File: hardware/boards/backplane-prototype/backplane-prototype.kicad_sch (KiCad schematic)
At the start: 16 parts, among them J1 DC_IN, J10 SLOT_3_IO, J11 SLOT_4_IO, J12 SLOT_5_IO, J13 SLOT_6_IO, J2 SLOT_1, J3 SLOT_2, J4 SLOT_3, J5 SLOT_4, J6 SLOT_5, J7 SLOT_6, J8 SLOT_1_IO, J9 SLOT_2_IO

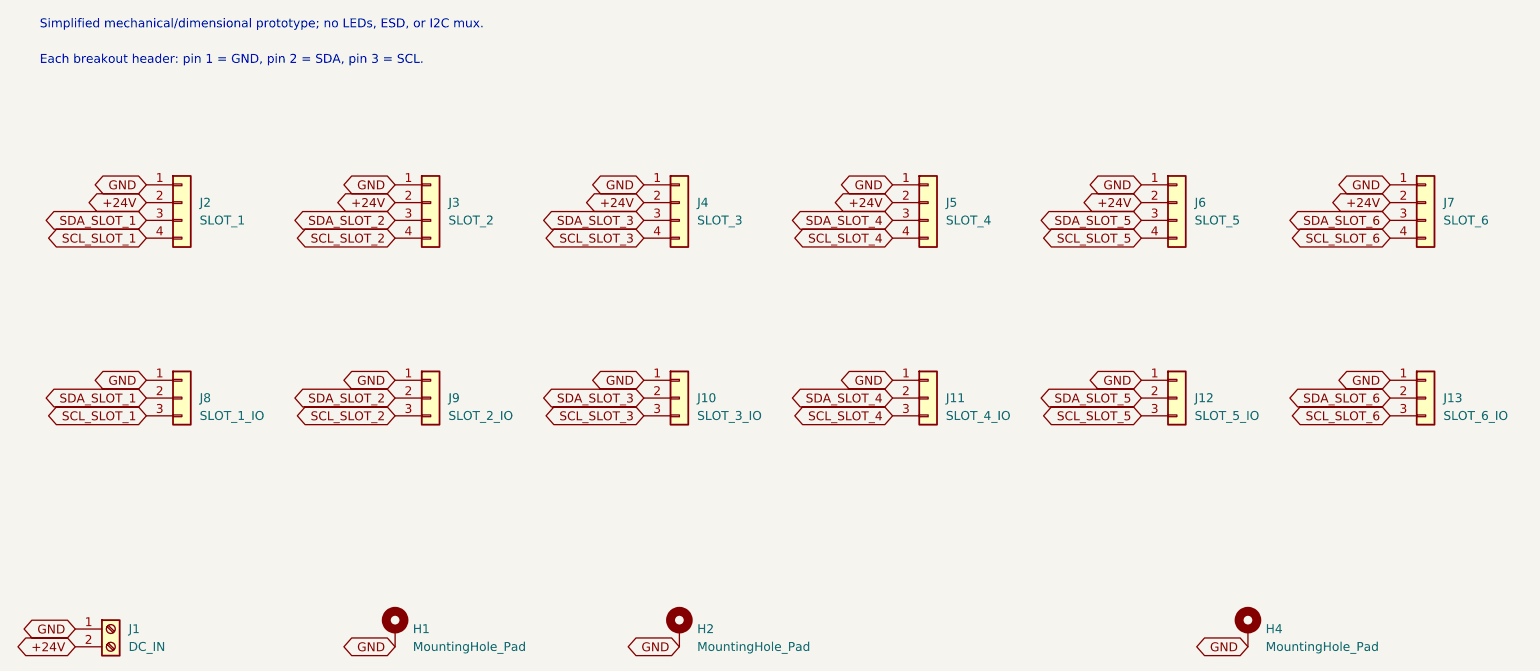
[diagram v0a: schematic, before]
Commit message: Checkpoint current hardware revisions
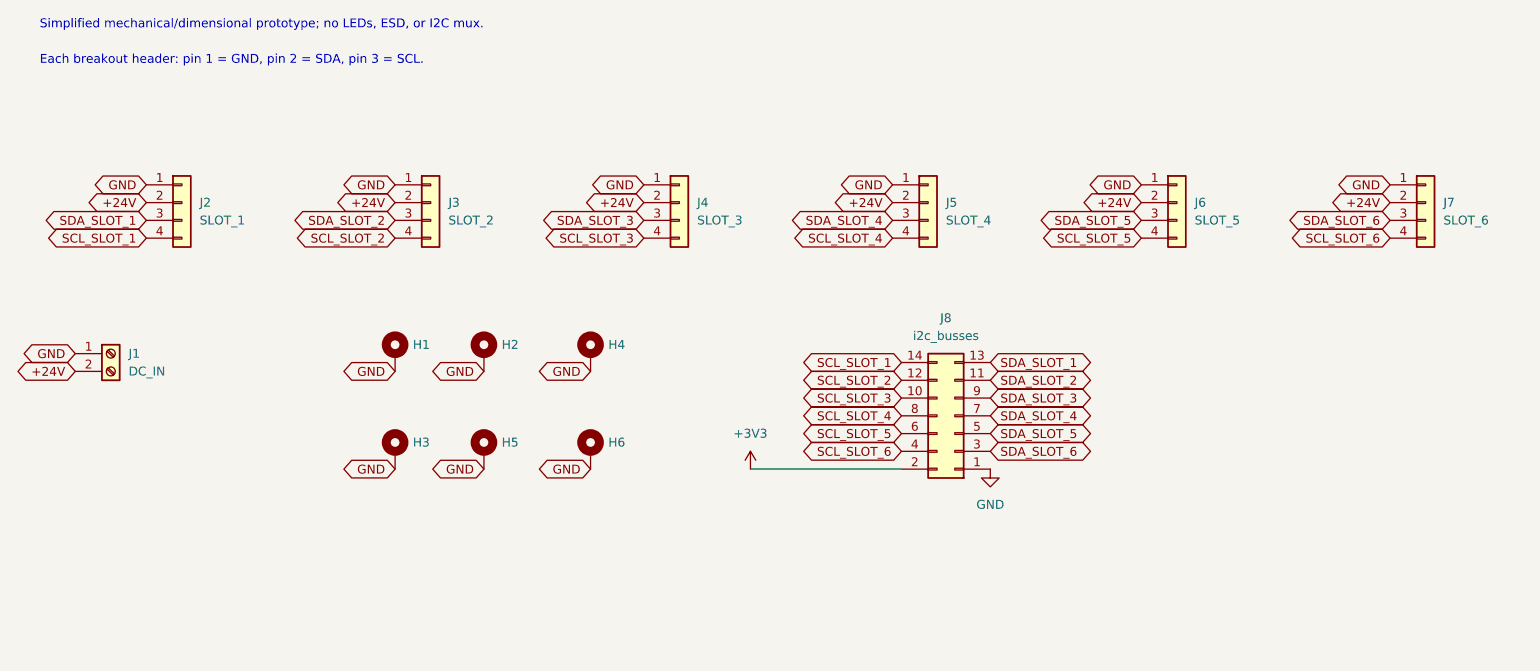
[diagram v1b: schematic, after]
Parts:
- removed J10: SLOT_3_IO, Connector_PinHeader_2.54mm:PinHeader_1x03_P2.54mm_Vertical, symbol Connector_Generic:Conn_01x03
- removed J11: SLOT_4_IO, Connector_PinHeader_2.54mm:PinHeader_1x03_P2.54mm_Vertical, symbol Connector_Generic:Conn_01x03
- removed J12: SLOT_5_IO, Connector_PinHeader_2.54mm:PinHeader_1x03_P2.54mm_Vertical, symbol Connector_Generic:Conn_01x03
- removed J13: SLOT_6_IO, Connector_PinHeader_2.54mm:PinHeader_1x03_P2.54mm_Vertical, symbol Connector_Generic:Conn_01x03
- removed J8: SLOT_1_IO, Connector_PinHeader_2.54mm:PinHeader_1x03_P2.54mm_Vertical, symbol Connector_Generic:Conn_01x03
- removed J9: SLOT_2_IO, Connector_PinHeader_2.54mm:PinHeader_1x03_P2.54mm_Vertical, symbol Connector_Generic:Conn_01x03
- added H3, H5, H6: MountingHole_Pad, MountingHole:MountingHole_2.2mm_M2_Pad_Via, symbol Mechanical:MountingHole_Pad
- added J8: i2c_busses, Connector_PinHeader_1.00mm:PinHeader_2x07_P1.00mm_Vertical, symbol Connector_Generic:Conn_02x07_Odd_Even
- H1, H2, H4: footprint MountingHole:MountingHole_3.2mm_M3_Pad_Via -> MountingHole:MountingHole_2.2mm_M2_Pad_Via
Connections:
- net GND: now also H3.1, H5.1, H6.1, J8.1 (Pin_1)
- net SCL_SLOT_1: now also J8.14 (Pin_14)
- net SCL_SLOT_2: now also J8.12 (Pin_12)
- net SCL_SLOT_3: now also J8.10 (Pin_10)
- net SCL_SLOT_4: now also J8.8 (Pin_8)
- net SCL_SLOT_5: now also J8.6 (Pin_6)
- net SCL_SLOT_6: now also J8.4 (Pin_4)
- net SDA_SLOT_1: now also J8.13 (Pin_13)
- net SDA_SLOT_2: now also J8.11 (Pin_11)
- net SDA_SLOT_3: now also J8.9 (Pin_9)
- net SDA_SLOT_4: now also J8.7 (Pin_7)
- net SDA_SLOT_5: now also J8.5 (Pin_5)
- net SDA_SLOT_6: now also J8.3 (Pin_3)
- new net +3V3: J8.2 (Pin_2)
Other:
- moved on the sheet: H1, H2, H4, J1
